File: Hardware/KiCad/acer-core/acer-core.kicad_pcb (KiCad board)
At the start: 4 copper layers, 31.5 x 36.9 mm, 19 parts, among them J1 Conn_01x14_Pin, J2 Conn_01x14_Pin, U1 ESP32-S3-WROOM-1-N4, U2 WIO-SX1262

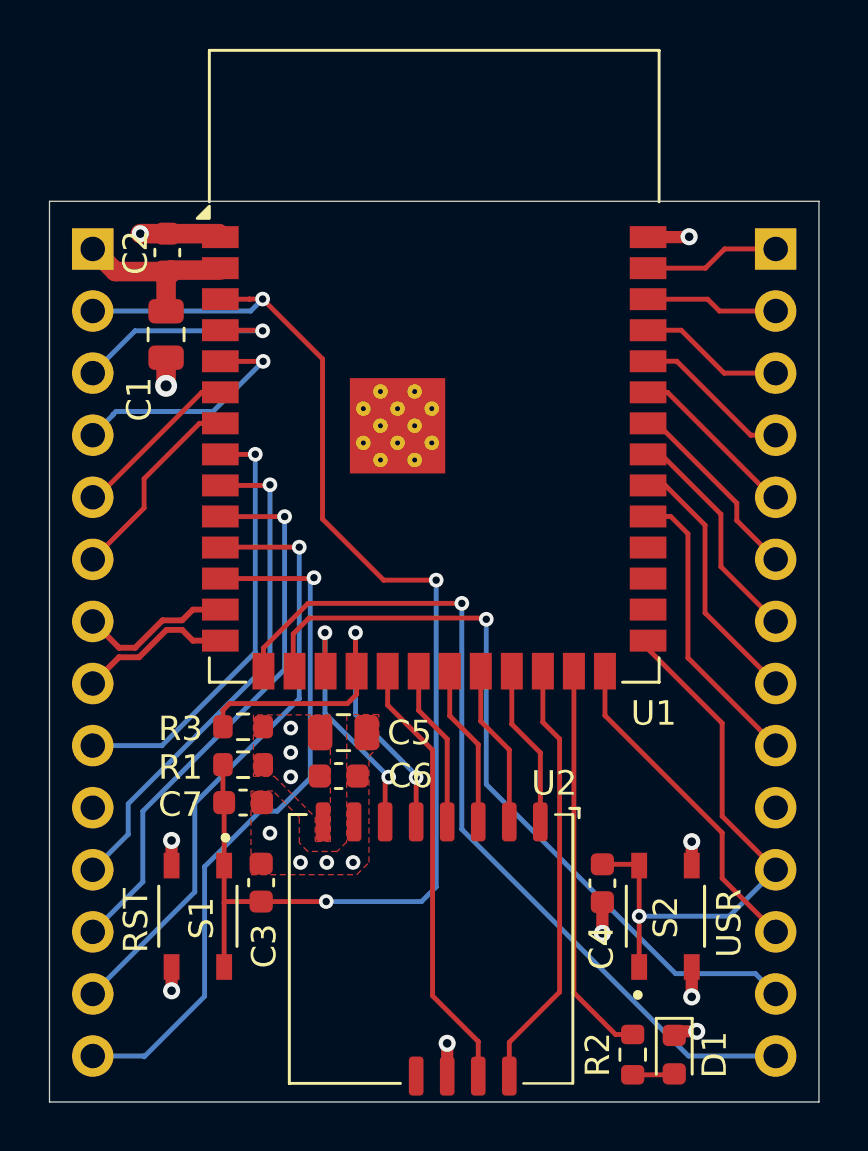
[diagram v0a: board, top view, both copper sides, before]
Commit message: Routing Done
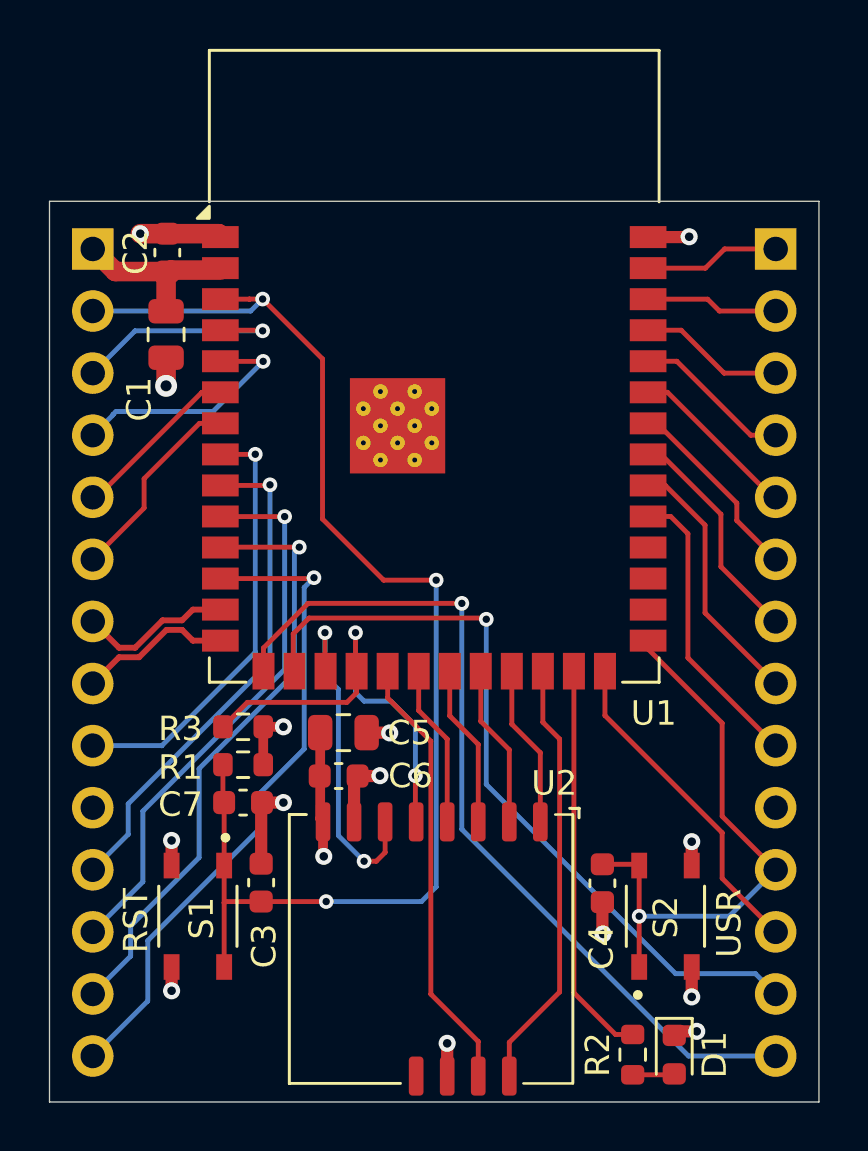
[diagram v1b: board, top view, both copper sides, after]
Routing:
- net +3.3V: track 7.37 -> 14.9 mm, vias 3 -> 2
- net GND: track 14.0 -> 21.2 mm, vias 14 -> 13
- net /LORA_NSS: track 10.5 -> 13.9 mm
- net /IO8: track 28.8 -> 27.2 mm
- removed copper zone on F.Cu, net +3.3V
- removed copper zone on F.Cu, net GND
